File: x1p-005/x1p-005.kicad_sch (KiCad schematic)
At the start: 38 parts, among them Q1 LMBT3904LT1G, SW1 6.0*6.0*6.0, SW2 6.0*6.0*6.0, U1 AD24C02, U2 SN74LVC1T45DBVR

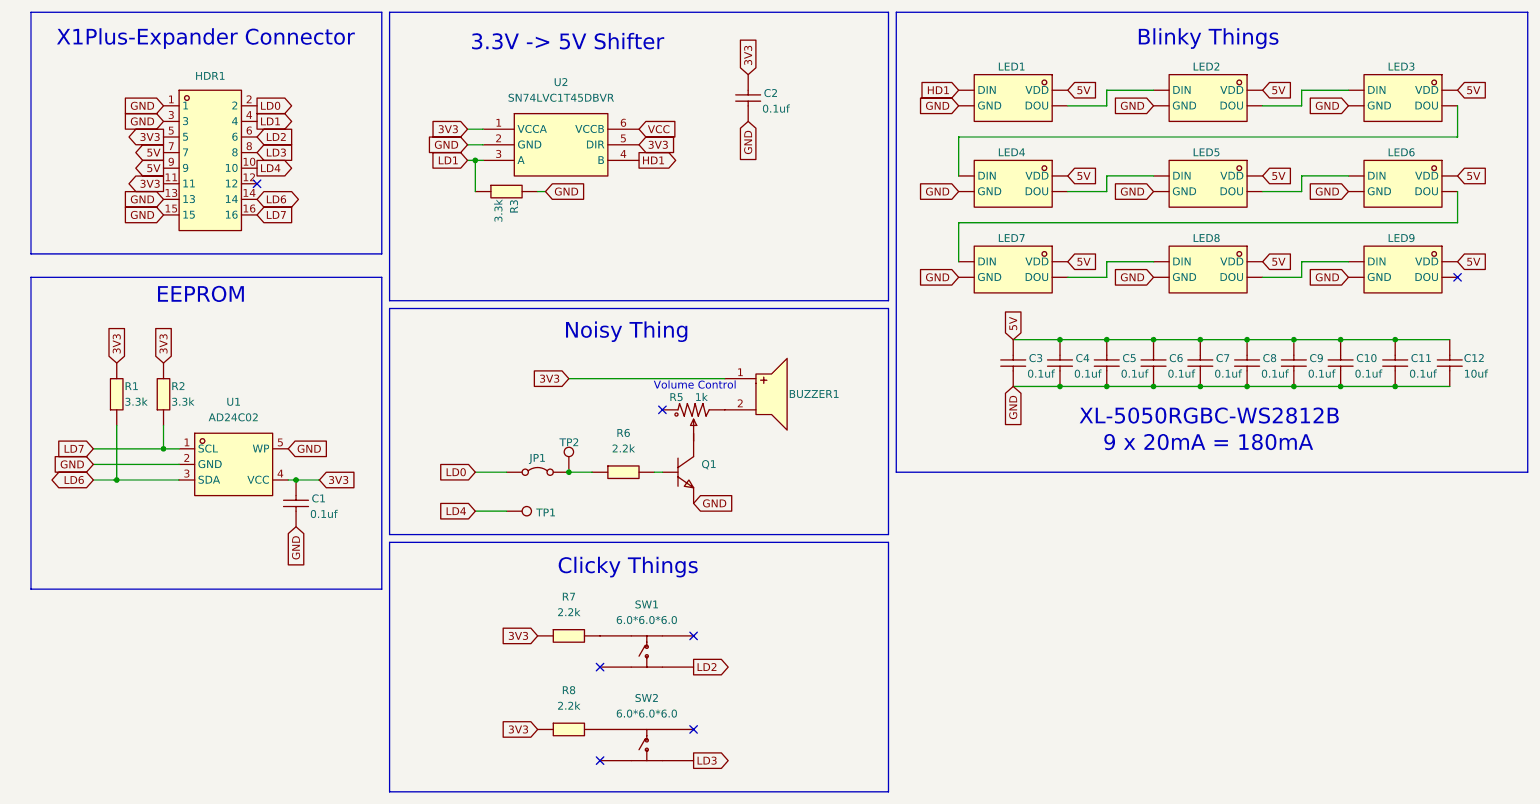
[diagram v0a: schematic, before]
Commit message: add eeprom/switch mux, change buzzer
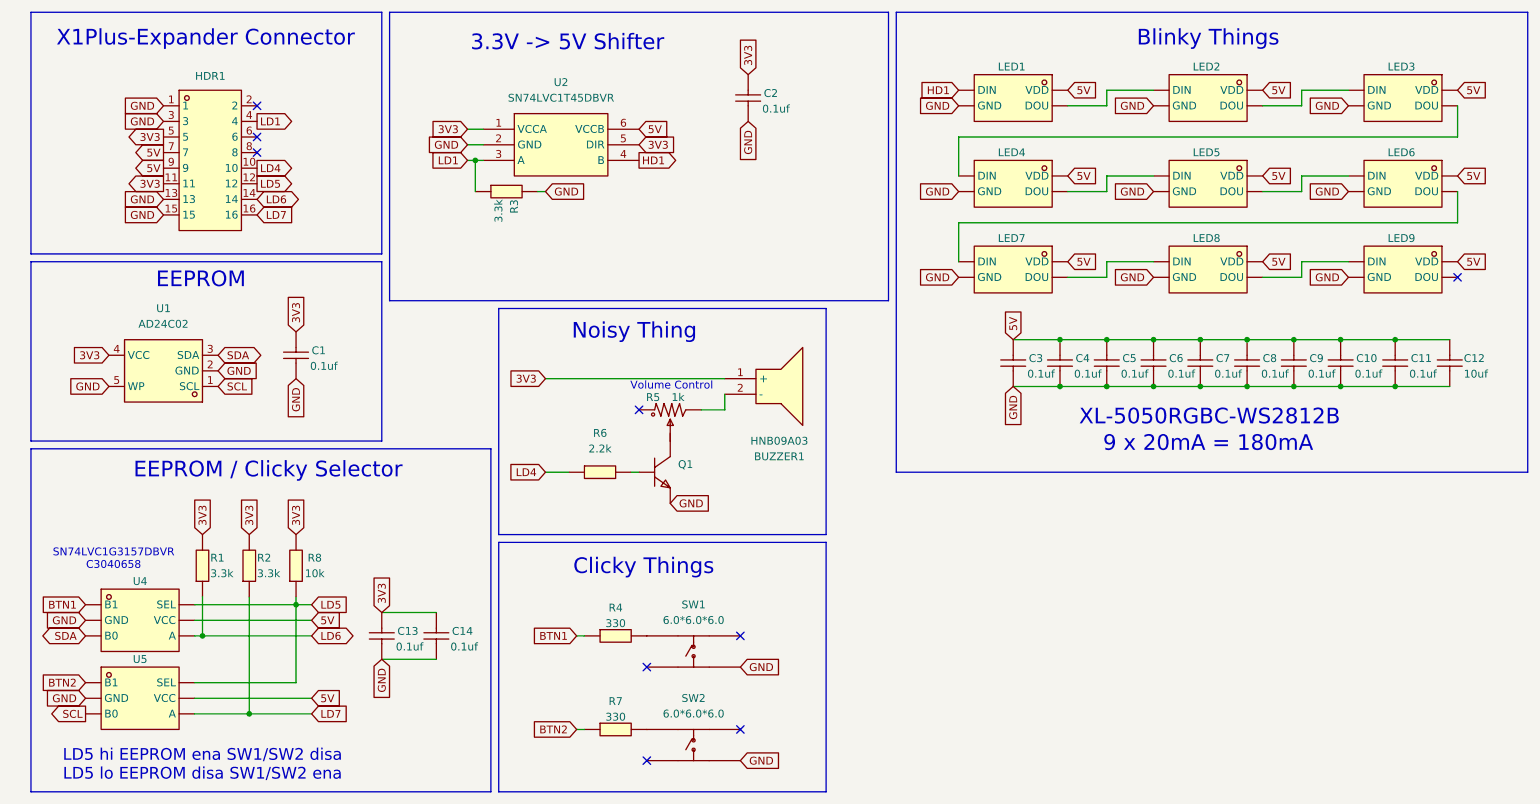
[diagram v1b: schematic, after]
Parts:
- removed BUZZER1: QMB-09B-03, x1p-005:BUZ-TH_BD9.0-P4.00-D0.6-FD, symbol x1p-005:QMB-09B-03
- removed JP1: Jumper_2_Bridged, Jumper:SolderJumper-2_P1.3mm_Bridged_RoundedPad1.0x1.5mm, symbol Jumper:Jumper_2_Bridged
- removed R7, R8: 2.2k, x1p-005:R0402, symbol x1p-005:0402WGF2201TCE
- removed TP1, TP2: TestPoint, TestPoint:TestPoint_Pad_D2.0mm, symbol Connector:TestPoint
- added BUZZER1: HNB09A03, x1p-005:BUZ-TH_BD9.0-P5.00-D0.6-FD, symbol x1p-005:HNB09A03
- added C13, C14: 0.1uf, x1p-005:C0402, symbol lcsc:CL05B104KO5NNNC
- added R4, R7: 330, x1p-005:R0402, symbol x1p-005:0402WGF3300TCE
- added R8: 10k, x1p-005:R0402, symbol x1p-005:0402WGF1002TCE
- added U4, U5: SN74LVC1G3157DBVR_C3040658, x1p-005:SOT-23-6_L2.9-W1.6-P0.95-LS2.8-BL, symbol x1p-005:SN74LVC1G3157DBVR_C3040658
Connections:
- net VCC is gone; now on net 5V: U2.6 (VCCB)
- net 3V3: now also BUZZER1.1 (+), C13.1, C14.1, R8.2
- net 5V: now also U4.5 (VCC), U5.5 (VCC)
- net GND: now also SW1.4, SW2.4, C13.2, C14.2, U4.2 (GND), U5.2 (GND)
- net LD4: now also R6.1
- net LD6: now also U4.4 (A); no longer U1.3 (SDA)
- net LD7: now also U5.4 (A); no longer U1.1 (SCL)
- net at R5.3: now also BUZZER1.2 (-)
- net LD5: now reaches HDR1.12
- net LD5: now also R8.1, U4.6 (SEL), U5.6 (SEL)
- net at SW1.1: now also R4.2
- net at SW2.1: now also R7.2
- net LD0: no longer names the net of HDR1.2
- net LD2: no longer names the net of HDR1.6
- net LD2: no longer SW1.4
- net LD3: no longer names the net of HDR1.8
- net LD3: no longer SW2.4
- new net BTN1: R4.1, U4.1 (B1)
- new net BTN2: R7.1, U5.1 (B1)
- new net SCL: U1.1 (SCL), U5.3 (B0)
- new net SDA: U1.3 (SDA), U4.3 (B0)
- no-connect marks 7 -> 9
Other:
- note added: "EEPROM / Clicky Selector"
- note added: "LD5 hi EEPROM ena SW1/SW2 disa LD5 lo EEPROM disa SW1/SW2 ena"
- note added: "SN74LVC1G3157DBVR C3040658"
- moved on the sheet: Q1, R5, R6, SW1, SW2

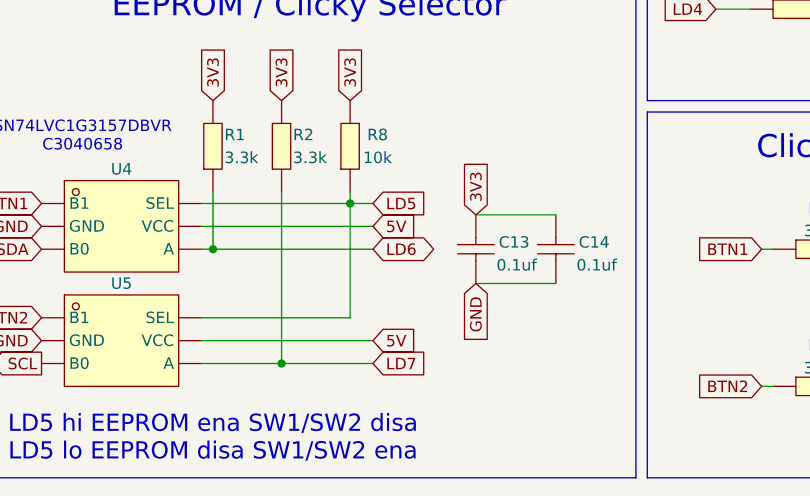
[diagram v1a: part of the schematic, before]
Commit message: 0 drc violations \o/
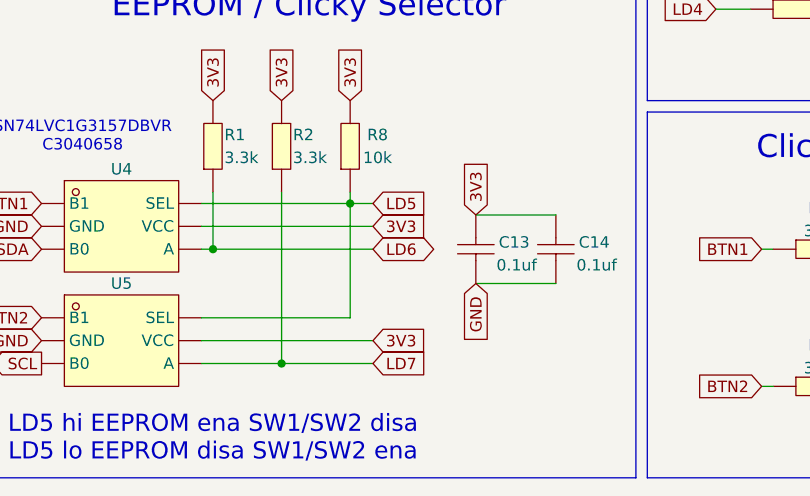
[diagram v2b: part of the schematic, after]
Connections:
- net 3V3: now also U4.5 (VCC), U5.5 (VCC)
- net 5V: no longer U4.5 (VCC), U5.5 (VCC)
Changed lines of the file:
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@@
+		)
+	)
+	(global_label "3V3"
+		(shape input)
+		(at 58.42 111.76 0)
+		(fields_autoplaced yes)
+		(effects
+			(font
+				(size 1.27 1.27)
+			)
+			(justify left)
+		)
+		(property "Intersheetrefs" "${INTERSHEET_REFS}"
+			(at 64.9128 111.76 0)
+			(effects
+				(font
+					(size 1.27 1.27)
+				)
+				(justify left)
+				(hide yes)
+			)
 		)
 	)
@@
 		)
 	)
-	(global_label "5V"
+	(global_label "3V3"
+		(shape input)
+		(at 48.26 97.79 90)
+		(fields_autoplaced yes)
+		(effects
+			(font
+				(size 1.27 1.27)
+			)
+			(justify left)
+		)
+		(property "Intersheetrefs" "${INTERSHEET_REFS}"
+			(at 48.26 91.2972 90)
+			(effects
+				(font
+					(size 1.27 1.27)
+				)
+				(justify left)
+				(hide yes)
+			)
+		)
+	)
+	(global_label "GND"
+		(shape input)
+		(at 129.54 30.48 270)
+		(fields_autoplaced yes)
+		(effects
+			(font
+				(size 1.27 1.27)
+			)
+			(justify right)
+		)
+		(property "Intersheetrefs" "${INTERSHEET_REFS}"
+			(at 129.54 37.3357 90)
+			(effects
+				(font
+					(size 1.27 1.27)
+				)
+				(justify right)
+				(hide yes)
+			)
+		)
+	)
+	(global_label "GND"
+		(shape input)
+		(at 34.29 43.18 180)
+		(fields_autoplaced yes)
+		(effects
+			(font
+				(size 1.27 1.27)
+			)
+			(justify right)
+		)
+		(property "Intersheetrefs" "${INTERSHEET_REFS}"
+			(at 27.4343 43.18 0)
+			(effects
+				(font
+					(size 1.27 1.27)
+				)
+				(justify right)
+				(hide yes)
+			)
+		)
+	)
+	(global_label "3V3"
 		(shape input)
 		(at 58.42 124.46 0)
@@
 		)
 		(property "Intersheetrefs" "${INTERSHEET_REFS}"
-			(at 63.7033 124.46 0)
-			(effects
-				(font
-					(size 1.27 1.27)
-				)
-				(justify left)
-				(hide yes)
-			)
-		)
-	)
-	(global_label "3V3"
-		(shape input)
-		(at 48.26 97.79 90)
-		(fields_autoplaced yes)
-		(effects
-			(font
-				(size 1.27 1.27)
-			)
-			(justify left)
-		)
-		(property "Intersheetrefs" "${INTERSHEET_REFS}"
-			(at 48.26 91.2972 90)
-			(effects
-				(font
-					(size 1.27 1.27)
-				)
-				(justify left)
-				(hide yes)
-			)
-		)
-	)
-	(global_label "GND"
-		(shape input)
-		(at 129.54 30.48 270)
-		(fields_autoplaced yes)
-		(effects
-			(font
-				(size 1.27 1.27)
-			)
-			(justify right)
-		)
-		(property "Intersheetrefs" "${INTERSHEET_REFS}"
-			(at 129.54 37.3357 90)
-			(effects
-				(font
-					(size 1.27 1.27)
-				)
-				(justify right)
-				(hide yes)
-			)
-		)
-	)
-	(global_label "GND"
-		(shape input)
-		(at 34.29 43.18 180)
-		(fields_autoplaced yes)
-		(effects
-			(font
-				(size 1.27 1.27)
-			)
-			(justify right)
-		)
-		(property "Intersheetrefs" "${INTERSHEET_REFS}"
-			(at 27.4343 43.18 0)
-			(effects
-				(font
-					(size 1.27 1.27)
-				)
-				(justify right)
-				(hide yes)
-			)
-		)
-	)
-	(global_label "5V"
-		(shape input)
-		(at 58.42 111.76 0)
-		(fields_autoplaced yes)
-		(effects
-			(font
-				(size 1.27 1.27)
-			)
-			(justify left)
-		)
-		(property "Intersheetrefs" "${INTERSHEET_REFS}"
-			(at 63.7033 111.76 0)
-			(effects
-				(font
+			(at 64.9128 124.46 0)
+			(effects
+				(font
